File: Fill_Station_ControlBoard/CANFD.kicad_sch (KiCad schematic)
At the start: 10 parts, among them J14 DE9_Socket_MountingHoles, U5 TCAN337G

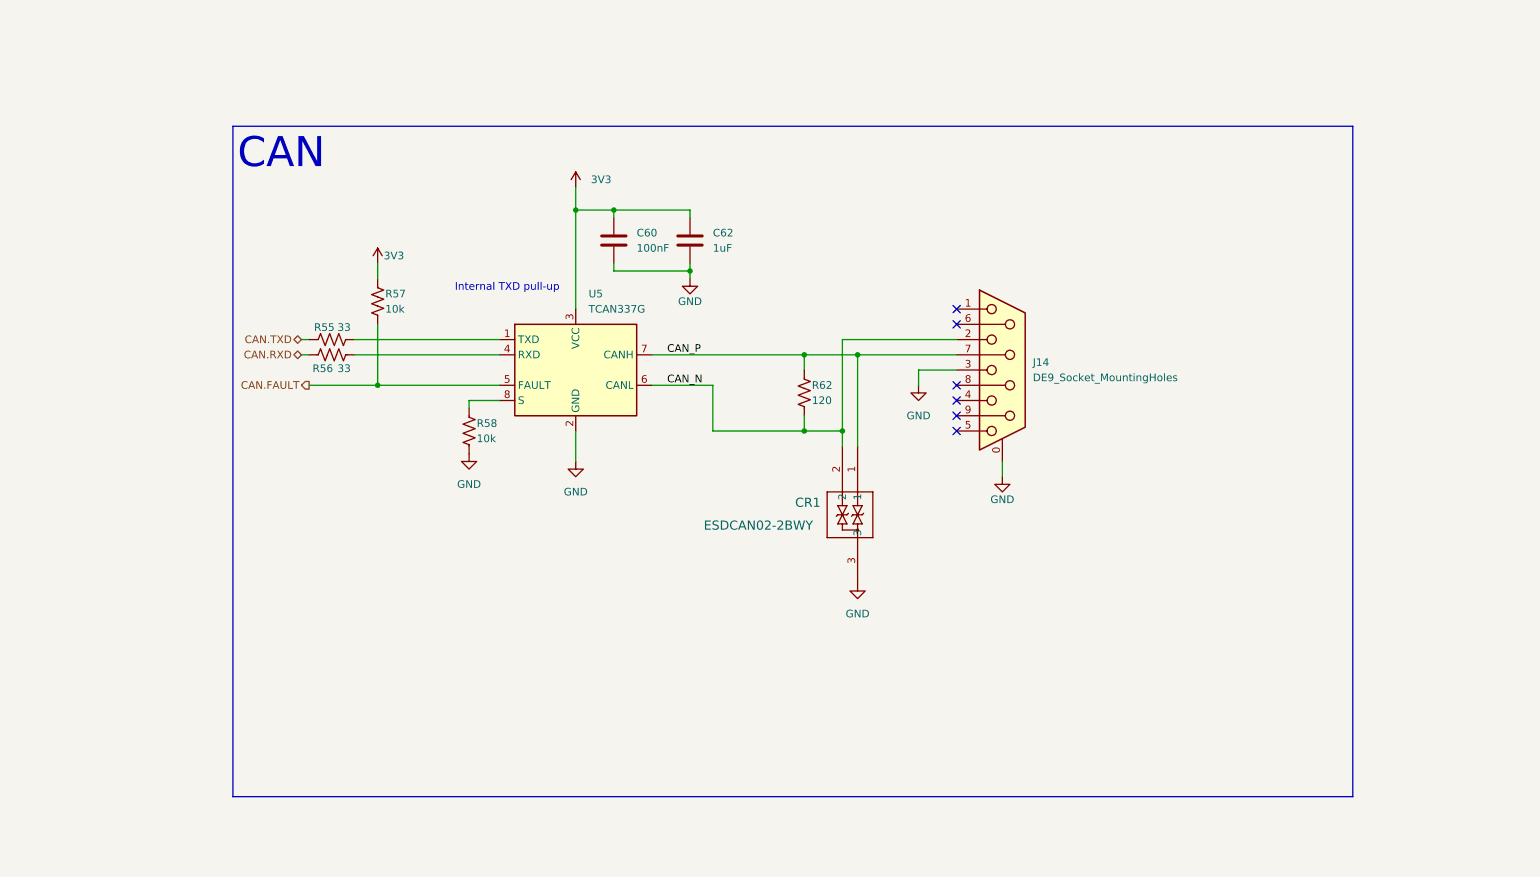
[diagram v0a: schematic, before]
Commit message: PCB fait
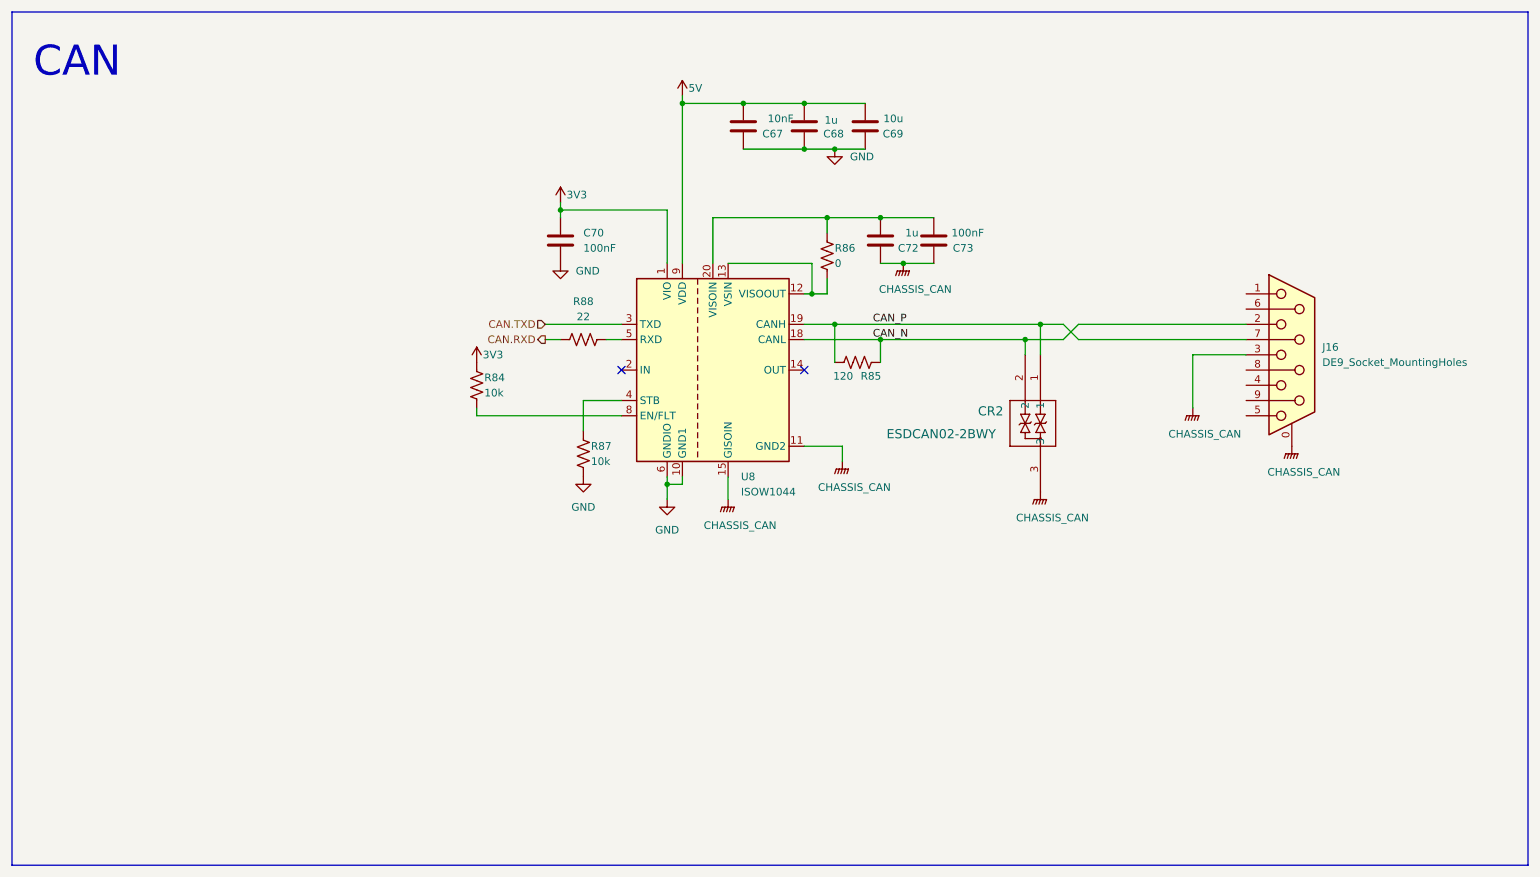
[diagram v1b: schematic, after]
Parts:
- removed C60: 100nF, Capacitor_SMD:C_0603_1608Metric, symbol Device:C
- removed C62: 1uF, Capacitor_SMD:C_0603_1608Metric, symbol Device:C
- removed CR1: ESDCAN02-2BWY, ESDCAN:SOT323-3L_STM, symbol ESDCAN:ESDCAN02-2BWY
- removed J14: DE9_Socket_MountingHoles, Connector_Dsub:DSUB-9_Socket_Vertical_P2.77x2.84mm_MountingHoles, symbol Connector:DE9_Socket_MountingHoles
- removed R55, R56: 33, Resistor_SMD:R_0603_1608Metric_Pad0.98x0.95mm_HandSolder, symbol Device:R_US
- removed R57, R58: 10k, Resistor_SMD:R_0603_1608Metric_Pad0.98x0.95mm_HandSolder, symbol Device:R_US
- removed R62: 120, Resistor_SMD:R_0603_1608Metric_Pad0.98x0.95mm_HandSolder, symbol Device:R_US
- removed U5: TCAN337G, Package_TO_SOT_SMD:TSOT-23-8_HandSoldering, symbol Interface_CAN_LIN:TCAN337G
- added C67: 10nF, Capacitor_SMD:C_0603_1608Metric, symbol Device:C
- added C68, C72: 1u, Capacitor_SMD:C_0603_1608Metric, symbol Device:C
- added C69: 10u, Capacitor_SMD:C_0603_1608Metric, symbol Device:C
- added C70, C73: 100nF, Capacitor_SMD:C_0603_1608Metric, symbol Device:C
- added CR2: ESDCAN02-2BWY, ESDCAN:SOT323-3L_STM, symbol ESDCAN:ESDCAN02-2BWY
- added J16: DE9_Socket_MountingHoles, Connector_Dsub:DSUB-9_Socket_Vertical_P2.77x2.84mm_MountingHoles, symbol Connector:DE9_Socket_MountingHoles
- added R84, R87: 10k, Resistor_SMD:R_0603_1608Metric_Pad0.98x0.95mm_HandSolder, symbol Device:R_US
- added R85: 120, Resistor_SMD:R_0603_1608Metric_Pad0.98x0.95mm_HandSolder, symbol Device:R_US
- added R86: 0, Resistor_SMD:R_0603_1608Metric_Pad0.98x0.95mm_HandSolder, symbol Device:R_US
- added R88: 22, Resistor_SMD:R_0402_1005Metric, symbol Device:R_US
- added U8: ISOW1044, Package_SO:SOIC-20W_7.5x12.8mm_P1.27mm, symbol Interface_CAN_LIN:ISOW1044
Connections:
- net 3V3: now also C70.1, R84.1, U8.1 (VIO)
- net CAN.RXD: now also R88.1
- net CAN.TXD: now also U8.3 (TXD)
- net CAN_N: now also CR2.2, J16.2, R85.1, U8.18 (CANL)
- net CAN_P: now also CR2.1, J16.7, R85.2, U8.19 (CANH)
- net GND: now also C67.1, C68.1, C69.1, C70.2, R87.2, U8.10 (GND1), U8.6 (GNDIO)
- new net: R88.2, U8.5 (RXD)
- new net: R86.2, U8.12 (VISOOUT), U8.13 (VSIN)
- new net: C72.2, C73.2, R86.1, U8.20 (VISOIN)
- new net: R87.1, U8.4 (STB)
- new net: R84.2, U8.8 (EN/FLT)
- new net 5V: C67.2, C68.2, C69.2, U8.9 (VDD)
- new net CHASSIS_CAN: C72.1, C73.1, CR2.3, J16.0 (PAD), J16.3, U8.11 (GND2), U8.15 (GISOIN), U8.16 (GISOIN), U8.17 (GISOIN)
- no-connect marks 6 -> 2
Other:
- note removed: "Internal TXD pull-up"
